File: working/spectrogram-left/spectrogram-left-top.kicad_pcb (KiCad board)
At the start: 2 copper layers, 146.1 x 111.2 mm, 7 parts

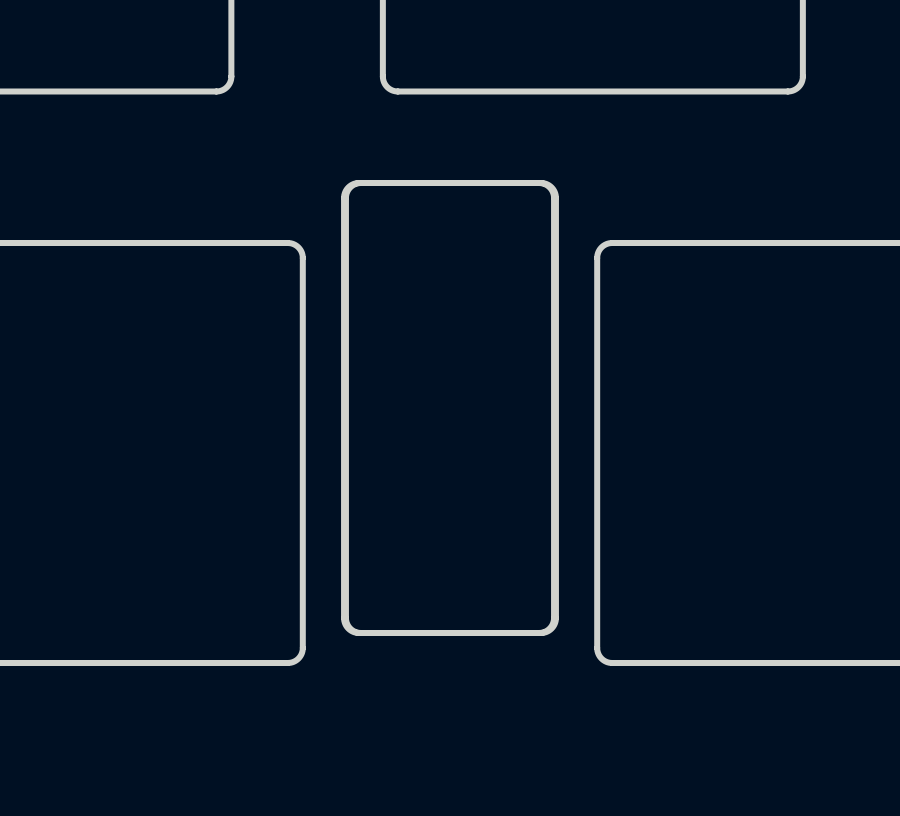
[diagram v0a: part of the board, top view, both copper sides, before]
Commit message: Pushed updtes
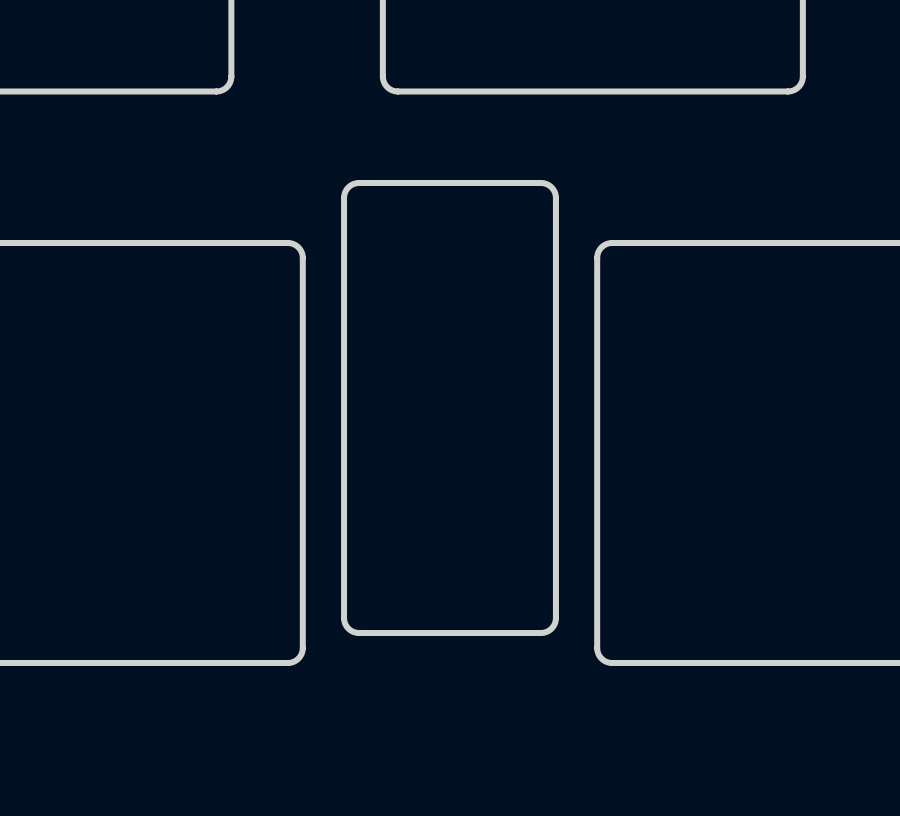
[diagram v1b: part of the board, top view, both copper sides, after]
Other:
- outline, holes or cut-outs redrawn
- net class Default removed
- net class Power Tracks removed
